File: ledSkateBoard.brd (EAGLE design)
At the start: 25.4 x 45.2 mm, 29 parts, among them J1 JST, U4 MIC2505 3.3

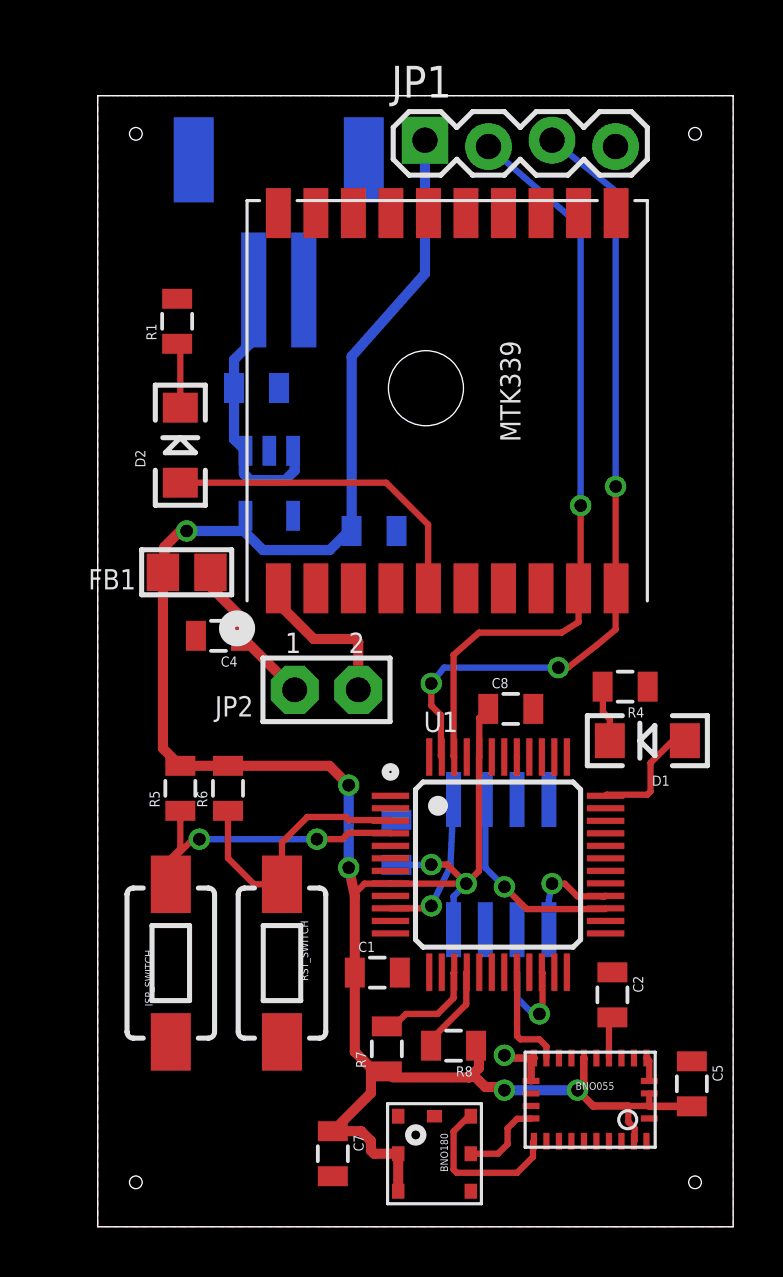
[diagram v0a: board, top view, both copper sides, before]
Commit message: Closer..
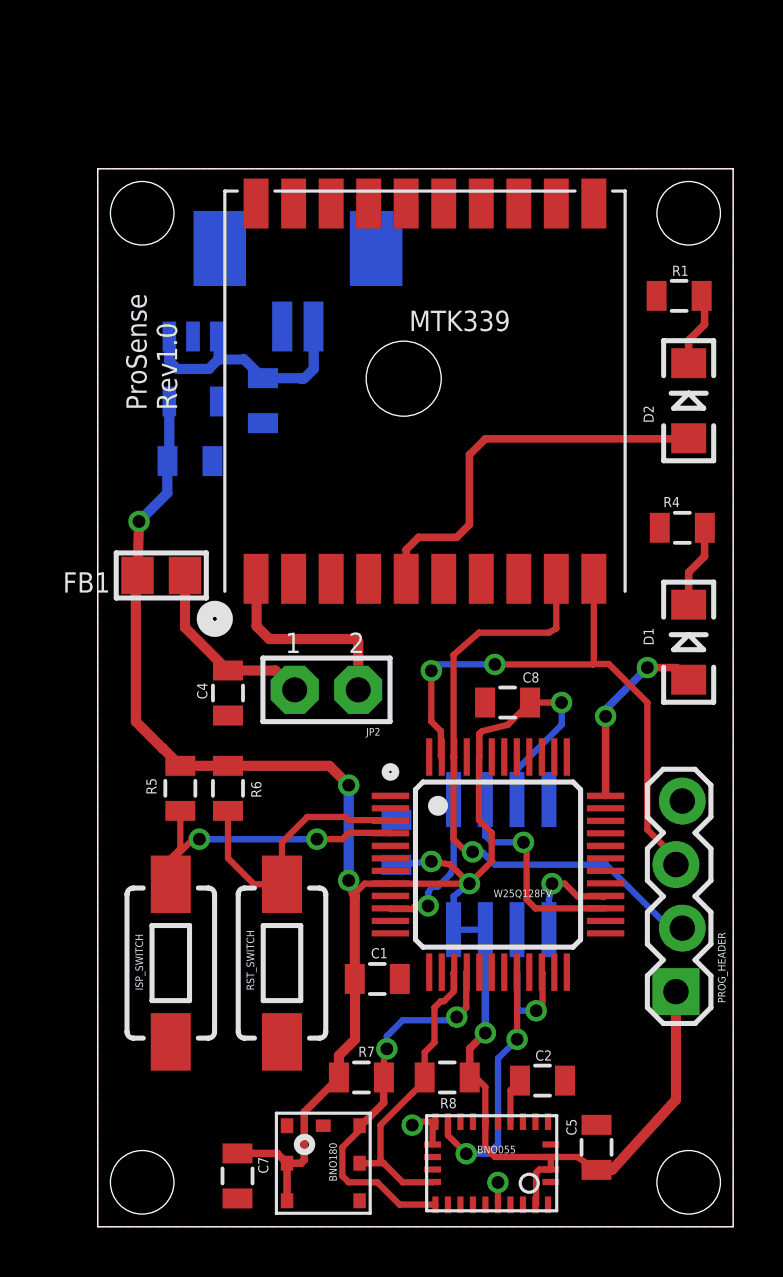
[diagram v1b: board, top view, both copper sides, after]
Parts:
- removed J1: JST, SparkFun-Connectors:JST-2-SMD
- removed JP1: (no value), SparkFun-Connectors:1X04_LOCK
- added BAT_CON: 53261-02, con-molex:53261-02
- added PROG_HEADER: (no value), SparkFun-Connectors:1X04_LOCK
- C15, C4, C8: value 10uF -> .1uF
- FB1: value (none) -> GetValue
- moved D2 20.4 mm to (59.2, 56.6)
- moved R1 20.1 mm to (58.8, 60.8), turned to 180 degrees
- moved C15 7.88 mm to (39.2, 54.2)
- moved R4 6.75 mm to (58.9, 51.6), turned to 0 degrees
- moved U4 5.49 mm to (39.4, 57.9)
- moved BNO055 4.69 mm to (51.3, 26.2)
- moved C5 4.58 mm to (55.5, 26.8)
- moved BNO180 4.46 mm to (44.6, 26.2)
- moved C2 4.42 mm to (53.3, 29.5), turned to 180 degrees
- moved D1 4.27 mm to (59.2, 47.0), turned to 90 degrees
- moved C7 3.91 mm to (41.1, 25.7)
- moved C4 2.32 mm to (40.8, 45.0), turned to 270 degrees
- moved R7 1.53 mm to (46.1, 29.6), turned to 0 degrees
- moved R8 1.30 mm to (49.5, 29.6)
- moved FB1 1.02 mm to (38.1, 49.7)
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- renumbered U1 to W25Q128FV
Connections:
- removed net N$5: R8.2, W25Q128FV.16
- removed net N$7: R4.1
- removed net N$8: R7.2, W25Q128FV.15
- removed net WS_RESET: U2.7
- net GND: now also BAT_CON.1, PROG_HEADER.4, R4.1; no longer J1.1, JP1.4
- net LPC_RX: now also PROG_HEADER.2; no longer JP1.2
- net LPC_TX: now also PROG_HEADER.3; no longer JP1.3
- net SCL: now also R8.2, W25Q128FV.15
- net SDA: now also R7.2, W25Q128FV.16
- net VCC: now also PROG_HEADER.1, U2.3, U2.7; no longer JP1.1
- net V_BATT: now also BAT_CON.2; no longer J1.2
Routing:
- net SDA: track 6.59 -> 15.6 mm, vias 0 -> 2
- net SCL: track 3.37 -> 12.2 mm
- net LPC_TX: track 32.1 -> 23.4 mm, vias 3 -> 2
- net BNO_INT: track 4.37 -> 10.2 mm, vias 0 -> 2
- net LPC_RX: track 30.3 -> 24.5 mm
- net N$8: track 4.18 -> 0.00 mm
- net N$5: track 3.50 -> 0.00 mm
- net N$1: track 4.75 -> 7.67 mm, vias 0 -> 2
- net N$6: track 13.2 -> 15.9 mm
- net N$10: track 6.35 -> 8.14 mm
- net VCC: track 97.2 -> 95.5 mm
- net N$4: track 6.09 -> 7.50 mm
- net V_BATT: track 11.2 -> 10.3 mm
- net N$3: track 2.76 -> 3.34 mm
- net GND: track 3.22 -> 3.00 mm, vias 1 -> 2
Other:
- board size 25.4 x 45.2 mm -> 25.4 x 42.3 mm
- board text added: "ProSense Rev1.0"
